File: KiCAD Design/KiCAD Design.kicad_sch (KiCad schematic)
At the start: 13 parts, among them SW1 SW_SPDT, U1 STM32F103C8Tx

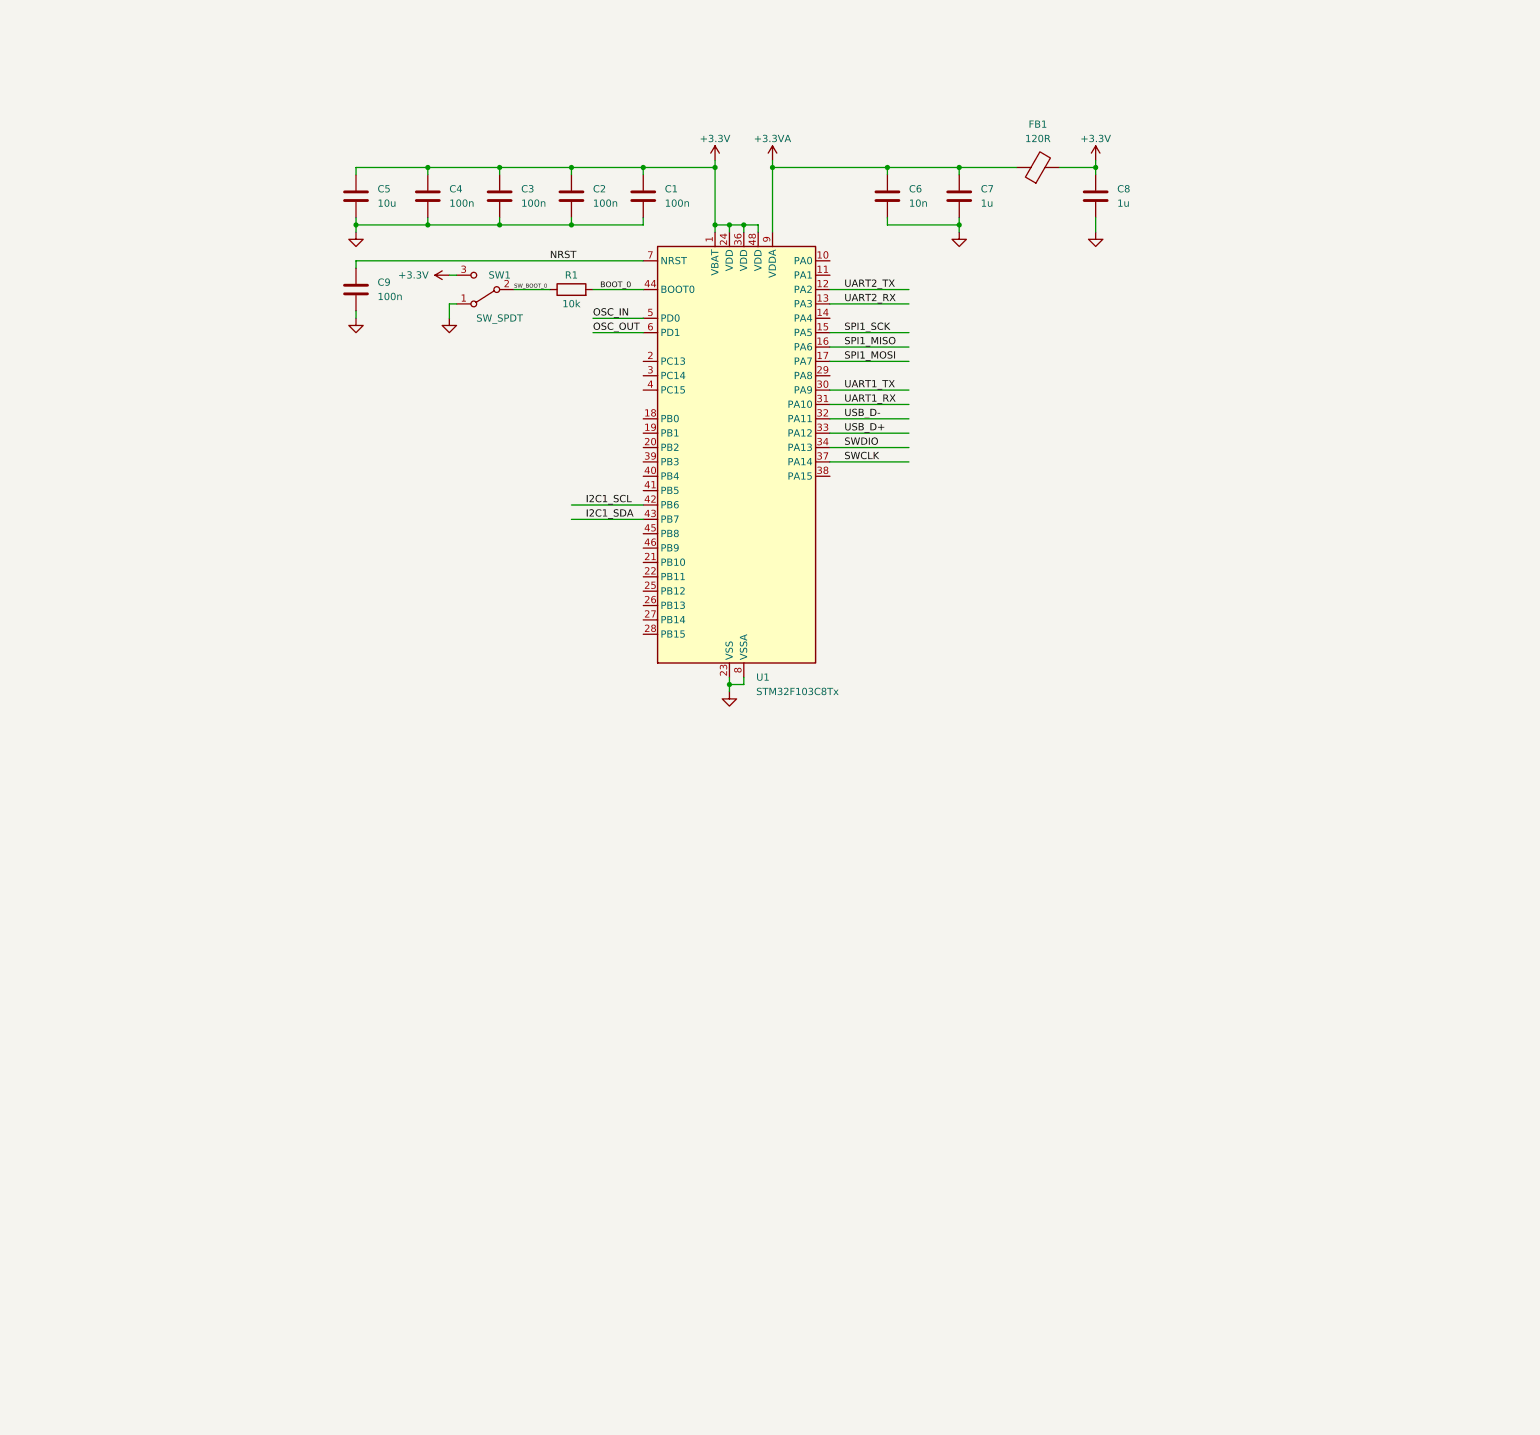
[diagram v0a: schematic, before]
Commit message: Kicad schematic work
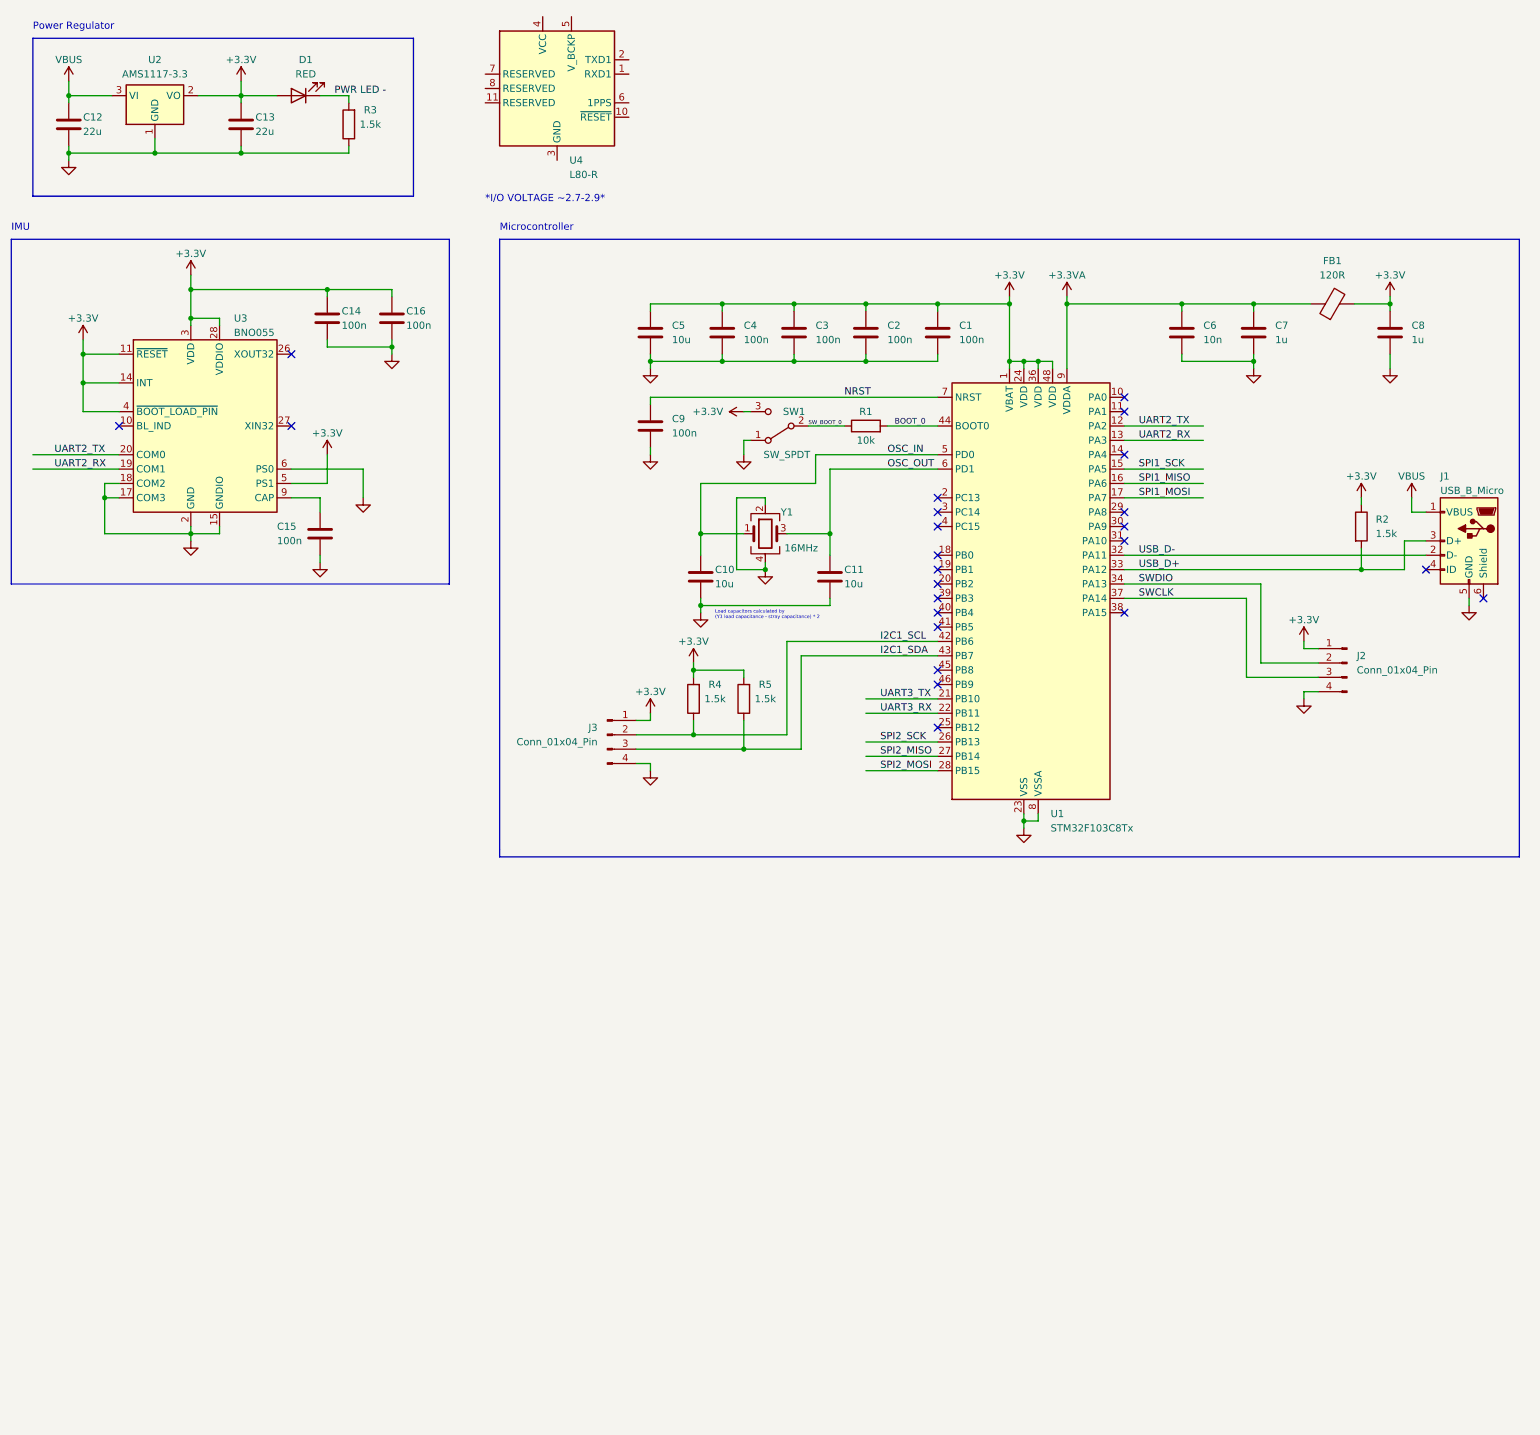
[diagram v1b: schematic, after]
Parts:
- added C10, C11: 10u, symbol Device:C
- added C12, C13: 22u, symbol Device:C
- added C14, C15, C16: 100n, symbol Device:C
- added D1: RED, symbol Device:LED
- added J1: USB_B_Micro, symbol Connector:USB_B_Micro
- added J2, J3: Conn_01x04_Pin, symbol Connector:Conn_01x04_Pin
- added R2, R3, R4, R5: 1.5k, symbol Device:R
- added U2: AMS1117-3.3, Package_TO_SOT_SMD:SOT-223-3_TabPin2, symbol Regulator_Linear:AMS1117-3.3
- added U3: BNO055, Package_LGA:LGA-28_5.2x3.8mm_P0.5mm, symbol Sensor_Motion:BNO055
- added U4: L80-R, RF_GPS:Quectel_L80-R, symbol RF_GPS:L80-R
- added Y1: 16MHz, symbol Device:Crystal_GND24
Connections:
- net +3.3V: now also C13.1, C14.2, C16.2, D1.2 (A), J2.1 (Pin_1), J3.1 (Pin_1), R2.1, R4.2, R5.2, U2.2 (VO), U3.11 (~{RESET}), U3.14 (INT), U3.28 (VDDIO), U3.3 (VDD), U3.4 (~{BOOT_LOAD_PIN}), U3.5 (PS1)
- net GND: now also C10.2, C11.2, C12.2, C13.2, C14.1, C15.1, C16.1, J1.5 (GND), J2.4 (Pin_4), J3.4 (Pin_4), R3.1, U2.1 (GND), U3.15 (GNDIO), U3.16 (GNDIO), U3.17 (COM3), U3.18 (COM2), U3.2 (GND), U3.25 (GNDIO), U3.6 (PS0), Y1.2, Y1.4
- net I2C1_SCL: now also J3.2 (Pin_2), R4.1
- net I2C1_SDA: now also J3.3 (Pin_3), R5.1
- net OSC_IN: now also C10.1, Y1.1
- net OSC_OUT: now also C11.1, Y1.3
- net SWCLK: now also J2.3 (Pin_3)
- net SWDIO: now also J2.2 (Pin_2)
- net UART2_RX: now also U3.19 (COM1)
- net UART2_TX: now also U3.20 (COM0)
- net USB_D+: now also J1.3 (D+), R2.2
- net USB_D-: now also J1.2 (D-)
- net UART3_TX: now reaches U1.21 (PB10)
- net UART3_RX: now reaches U1.22 (PB11)
- net SPI2_SCK: now reaches U1.26 (PB13)
- net SPI2_MISO: now reaches U1.27 (PB14)
- net SPI2_MOSI: now reaches U1.28 (PB15)
- net UART1_RX: no longer names the net of U1.31 (PA10)
- net UART1_TX: no longer names the net of U1.30 (PA9)
- new net: C15.2, U3.9 (CAP)
- new net: U4.12 (GND), U4.3 (GND)
- new net PWR LED -: D1.1 (K), R3.2
- new net VBUS: C12.1, J1.1 (VBUS), U2.3 (VI)
- no-connect marks 0 -> 24
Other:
- note added: "*I/O VOLTAGE ~2.7-2.9*"
- note added: "IMU"
- note added: "Load capacitors calculated by (Y1 load capacitance - stray capacitance) * 2"
- note added: "Microcontroller"
- note added: "Power Regulator"
- moved on the sheet: C1, C2, C3, C4, C5, C6, C7, C8, C9, FB1, R1, SW1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

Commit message: Some stuff
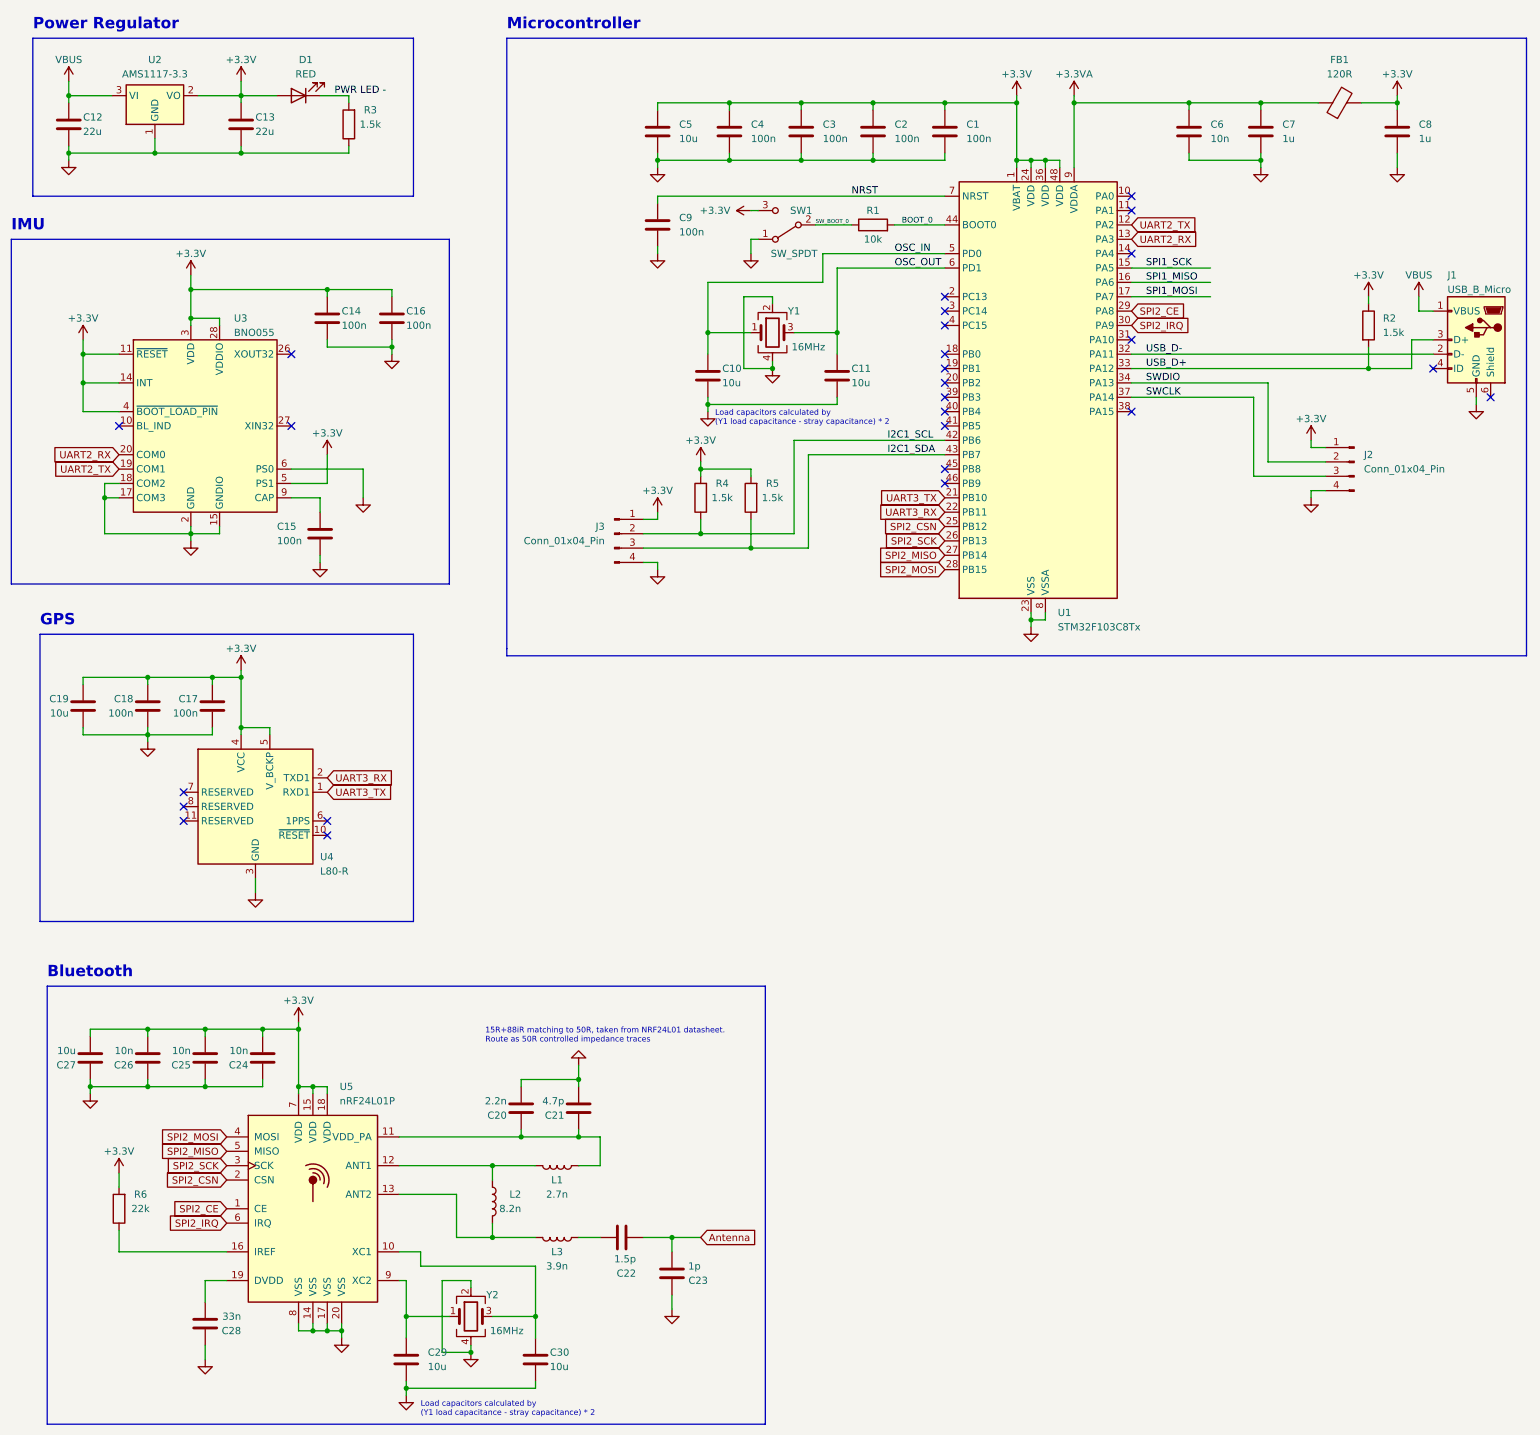
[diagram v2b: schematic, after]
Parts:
- added C17, C18: 100n, symbol Device:C
- added C19, C27, C29, C30: 10u, symbol Device:C
- added C20: 2.2n, symbol Device:C
- added C21: 4.7p, symbol Device:C
- added C22: 1.5p, symbol Device:C
- added C23: 1p, symbol Device:C
- added C24, C25, C26: 10n, symbol Device:C
- added C28: 33n, symbol Device:C
- added L1: 2.7n, symbol Device:L
- added L2: 8.2n, symbol Device:L
- added L3: 3.9n, symbol Device:L
- added R6: 22k, symbol Device:R
- added U5: nRF24L01P, Package_DFN_QFN:QFN-20-1EP_4x4mm_P0.5mm_EP2.5x2.5mm, symbol RF:nRF24L01P
- added Y2: 16MHz, symbol Device:Crystal_GND24
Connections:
- net +3.3V: now also U4.4 (VCC), U4.5 (V_BCKP), C17.2, C18.2, C19.2, C24.1, C25.1, C26.1, C27.1, R6.2, U5.15 (VDD), U5.18 (VDD), U5.7 (VDD)
- net GND: now also U4.12 (GND), U4.3 (GND), C17.1, C18.1, C19.1, C20.1, C21.1, C23.2, C24.2, C25.2, C26.2, C27.2, C28.2, C29.2, C30.2, U5.14 (VSS), U5.17 (VSS), U5.20 (VSS), U5.8 (VSS), Y2.2, Y2.4
- net SPI2_MISO: now also U5.5 (MISO)
- net SPI2_MOSI: now also U5.4 (MOSI)
- net SPI2_SCK: now also U5.3 (SCK)
- net UART2_RX: now also U3.20 (COM0); no longer U3.19 (COM1)
- net UART2_TX: now also U3.19 (COM1); no longer U3.20 (COM0)
- net UART3_RX: now also U4.2 (TXD1)
- net UART3_TX: now also U4.1 (RXD1)
- net SPI2_CSN: now reaches U1.25 (PB12)
- net SPI2_CSN: now also U5.2 (CSN)
- net SPI2_CE: now reaches U1.29 (PA8)
- net SPI2_CE: now also U5.1 (CE)
- net SPI2_IRQ: now reaches U1.30 (PA9)
- net SPI2_IRQ: now also U5.6 (IRQ)
- new net: C29.1, U5.9 (XC2), Y2.1
- new net: C30.1, U5.10 (XC1), Y2.3
- new net: C20.2, C21.2, L1.2, U5.11 (VDD_PA)
- new net: L1.1, L2.2, U5.12 (ANT1)
- new net: L2.1, L3.1, U5.13 (ANT2)
- new net: R6.1, U5.16 (IREF)
- new net: C28.1, U5.19 (DVDD)
- new net: C22.2, L3.2
- new net Antenna: C22.1, C23.1
- no-connect marks 24 -> 26
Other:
- note added: "15R+88iR matching to 50R, taken from NRF24L01 datasheet. Route as 50R controlled impedance traces"
- note added: "Bluetooth"
- note added: "GPS"
- note removed: "*I/O VOLTAGE ~2.7-2.9*"
- moved on the sheet: C1, C10, C11, C2, C3, C4, C5, C6, C7, C8, C9, FB1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
